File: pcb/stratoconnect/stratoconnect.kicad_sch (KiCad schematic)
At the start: 42 parts, among them J1 Conn_Coaxial, J2 Conn_02x03_Odd_Even, J3 Conn_01x04_Pin, J4 Conn_01x02_Pin, J5 Conn_01x05_Pin, SW1 SW_SPST, SW2 SW_SPST, U1 TPS565242, U2 ATmega328PB-A, U4 RF4463F30, Y1 CSTNE16M0V530000R0

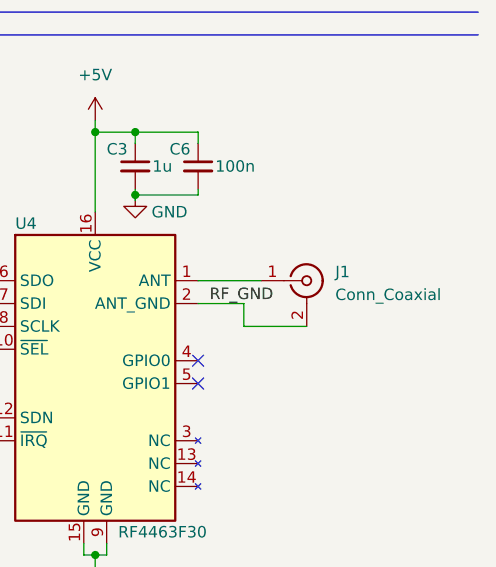
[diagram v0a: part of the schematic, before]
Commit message: WIP
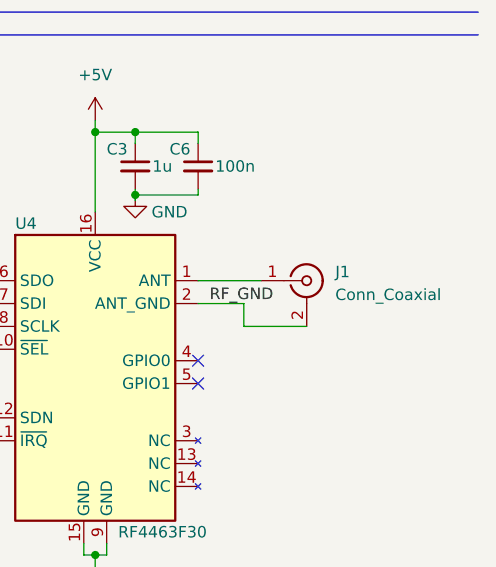
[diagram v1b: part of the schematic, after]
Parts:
- J1: footprint Connector_Coaxial:SMA_Molex_73251-2120_EdgeMount_Horizontal -> Connector_Coaxial:SMA_Amphenol_901-143_Horizontal
- J4: footprint (none) -> Connector_JST:JST_SH_BM04B-SRSS-TB_1x04-1MP_P1.00mm_Vertical
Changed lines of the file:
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@@
       (effects (font (size 1.27 1.27)))
     )
-    (property "Footprint" "" (at 153.67 100.33 0)
+    (property "Footprint" "Connector_JST:JST_SH_BM04B-SRSS-TB_1x04-1MP_P1.00mm_Vertical" (at 153.67 100.33 0)
       (effects (font (size 1.27 1.27)) hide)
     )
@@
   (symbol (lib_id "Connector:Conn_Coaxial") (at 266.065 110.49 0) (unit 1)
     (in_bom yes) (on_board yes) (dnp no) (fields_autoplaced)
-    (property "Reference" "J1" (at 269.24 109.5131 0)
-      (effects (font (size 1.27 1.27)) (justify left))
-    )
-    (property "Value" "Conn_Coaxial" (at 269.24 112.0531 0)
-      (effects (font (size 1.27 1.27)) (justify left))
-    )
-    (property "Footprint" "Connector_Coaxial:SMA_Molex_73251-2120_EdgeMount_Horizontal" (at 266.065 110.49 0)
-      (effects (font (size 1.27 1.27)) hide)
-    )
+    (property "Reference" "J1" (at 269.24 109.5132 0)
+      (effects (font (size 1.27 1.27)) (justify left))
+    )
+    (property "Value" "Conn_Coaxial" (at 269.24 112.0532 0)
+      (effects (font (size 1.27 1.27)) (justify left))
+    )
+    (property "Footprint" "Connector_Coaxial:SMA_Amphenol_901-143_Horizontal" (at 266.065 110.49 0)
+      (effects (font (size 1.27 1.27)) hide)
+    )
